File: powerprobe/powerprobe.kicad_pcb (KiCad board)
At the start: 2 copper layers, 41 parts, among them SW3 OS103011MS8QP1, U1 LT3045EMSE-PBF, U2 OPA847xD, U3 LT3045EMSE-PBF, U4 LT3094EMSE-TRPBF

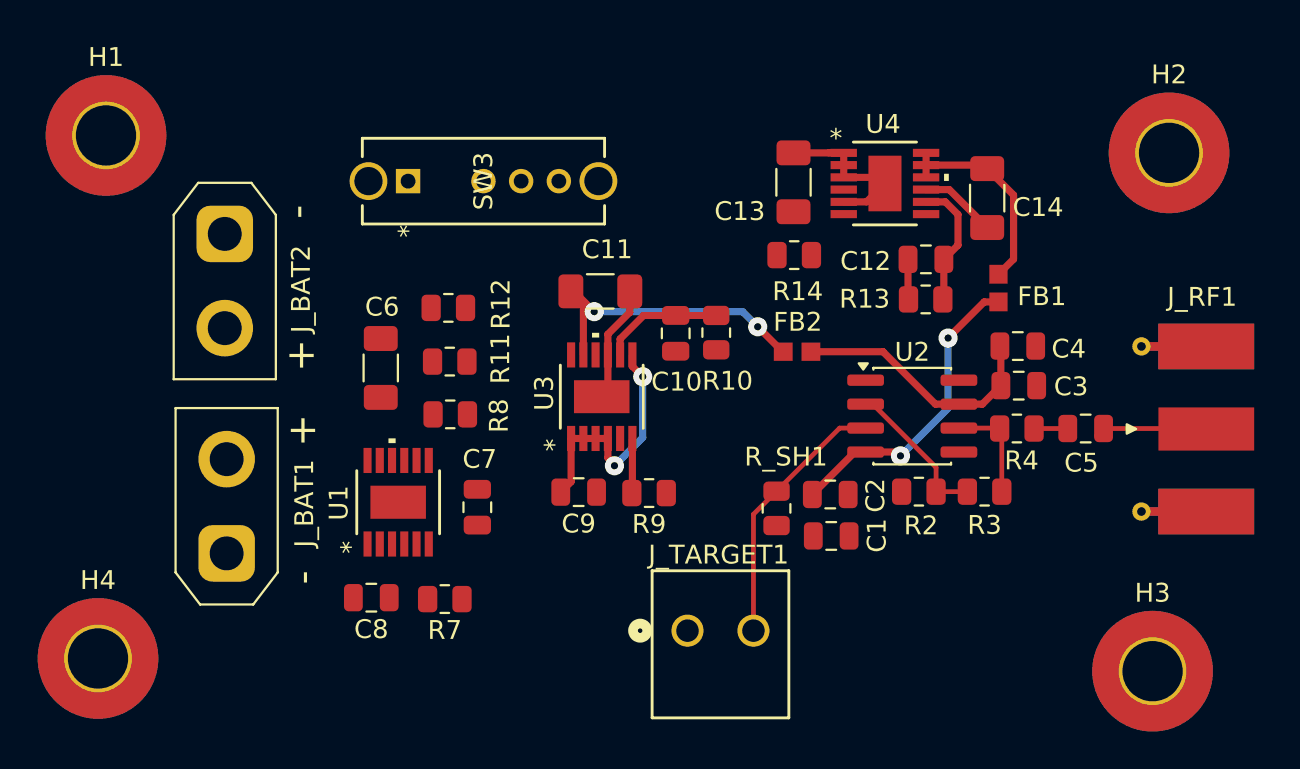
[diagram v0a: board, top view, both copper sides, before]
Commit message: Board finished
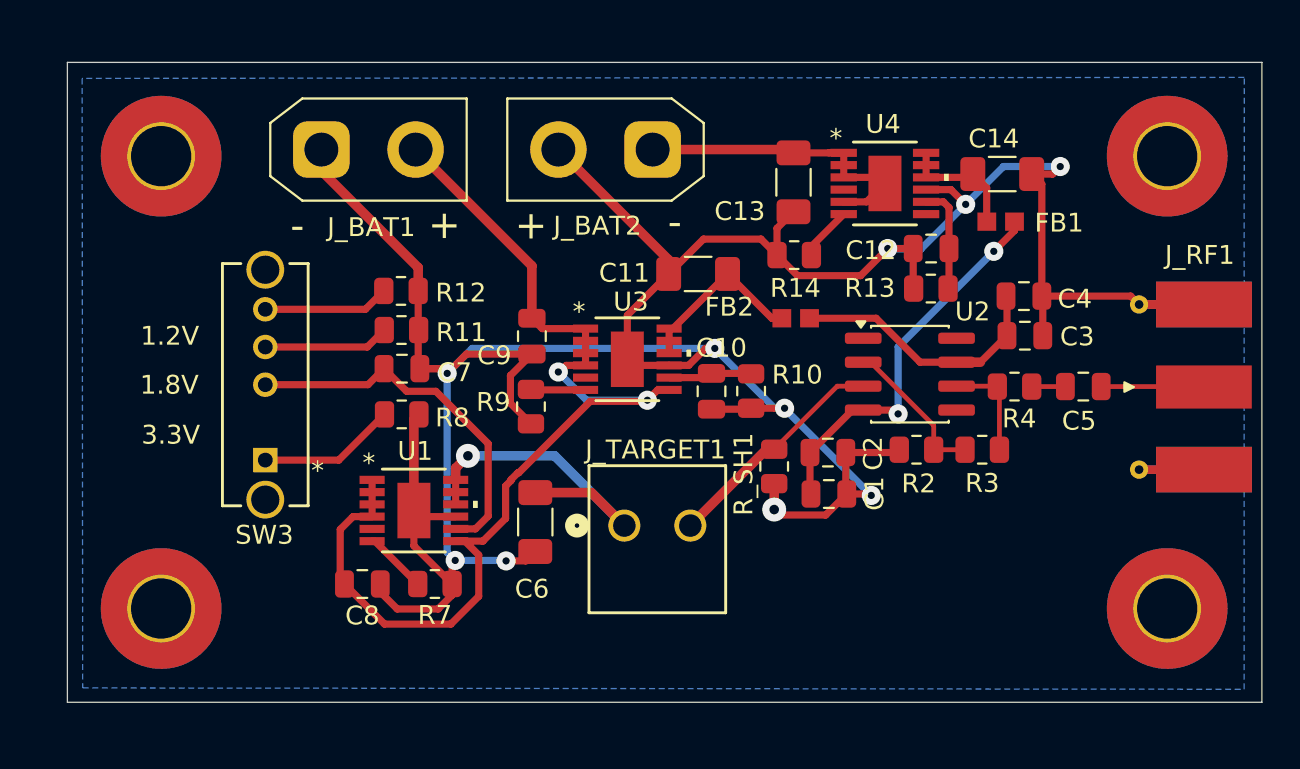
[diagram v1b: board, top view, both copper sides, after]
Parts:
- moved J_BAT2 23.1 mm to (164.5, 72.8), turned to 180 degrees
- moved J_BAT1 22.0 mm to (146.9, 72.8), turned to 0 degrees
- moved SW3 16.6 mm to (143.9, 89.3), turned to 180 degrees
- moved C6 11.6 mm to (158.2, 92.6), turned to 90 degrees
- moved C9 8.64 mm to (158.1, 82.7), turned to 90 degrees
- moved C7 8.37 mm to (151.2, 84.5), turned to 180 degrees
- moved R9 7.77 mm to (158.0, 86.5), turned to 90 degrees
- moved J_TARGET1 6.50 mm to (163.0, 92.8)
- moved C11 5.27 mm to (166.9, 79.4), turned to 0 degrees
- moved H4 4.27 mm to (138.4, 97.2)
- moved C10 3.61 mm to (167.6, 85.7)
- moved R10 3.61 mm to (169.7, 85.6)
- moved FB1 3.53 mm to (182.9, 76.7), turned to 180 degrees
- moved H3 3.41 mm to (191.8, 97.2)
- moved H1 3.13 mm to (138.4, 73.2)
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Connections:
- U1 pad 10: Net-(U1-OUTS) -> V_TARGET
- U1 pad 12: Net-(U1-OUTS) -> V_TARGET
- U3 pad 10: Net-(U3-OUTS) -> 5V
- U3 pad 12: Net-(U3-OUTS) -> 5V
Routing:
- net GND: track 12.4 -> 172.4 mm, vias 0 -> 10
- net /V_BAT+: track 13.3 -> 58.4 mm
- net /R_VT: track 0.00 -> 19.7 mm
- net V_TARGET: track 0.00 -> 18.1 mm, vias 0 -> 1
- net /V_BAT-: track 8.87 -> 16.4 mm
- net /R_3V3: track 0.00 -> 7.33 mm
- net /R_1V2: track 0.00 -> 6.69 mm
- net /R_1V8: track 0.00 -> 6.69 mm
- net 5V: track 16.2 -> 9.56 mm, vias 2 -> 0
- net -5V: track 11.3 -> 6.68 mm
- net Net-(U2-V-): track 16.5 -> 20.7 mm
- net Net-(U1-ILIM): track 0.00 -> 3.45 mm
- net Net-(U4-ILIM): track 0.03 -> 2.89 mm
- net Net-(U3-SET): track 6.46 -> 4.45 mm
- net VSS_TARGET: track 14.0 -> 12.2 mm
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- added copper zone on B.Cu, net GND
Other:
- board outline added: 63.4 x 34 mm
- board text added: "1.2V"
- board text added: "1.8V"
- board text added: "3.3V"
